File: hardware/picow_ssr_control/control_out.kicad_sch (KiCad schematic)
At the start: 12 parts

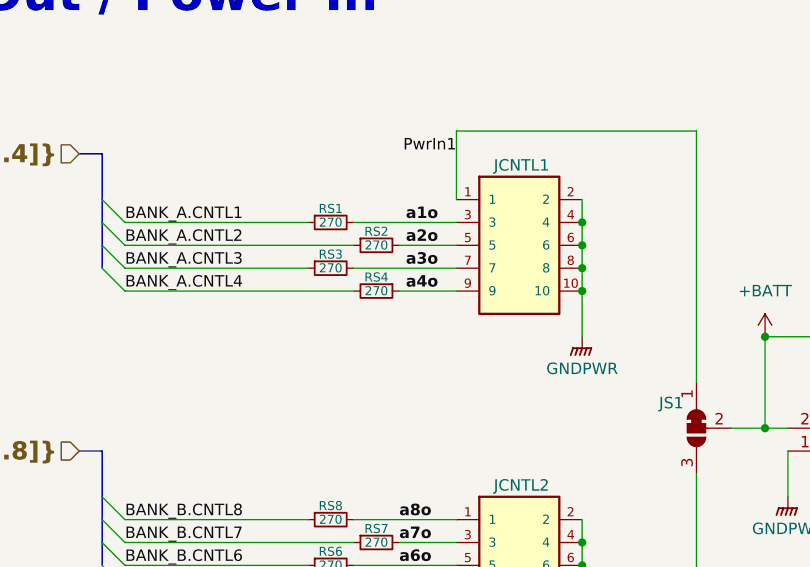
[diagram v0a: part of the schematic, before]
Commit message: Updated schemas
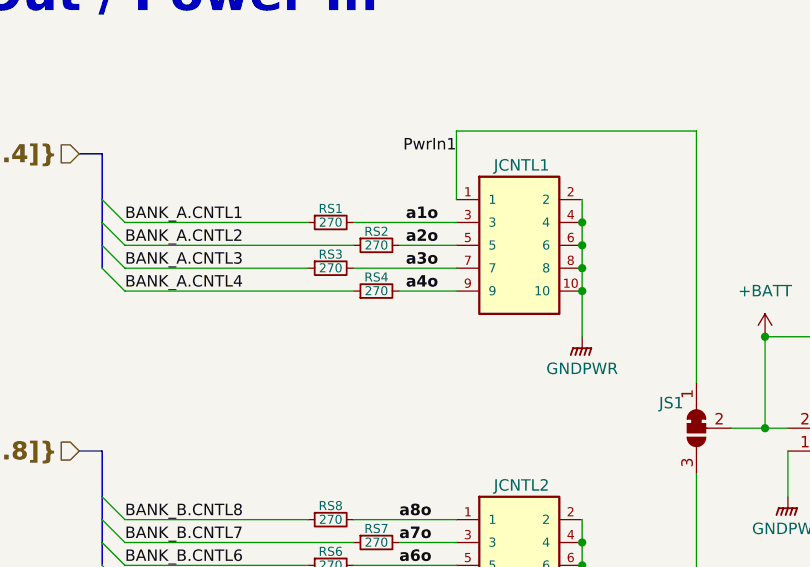
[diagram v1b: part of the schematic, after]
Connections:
- net BANK_A.CNTL4: now also RS4.1; no longer RS4.2
- net a4o: now also RS4.2; no longer RS4.1
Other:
- moved on the sheet: RS4
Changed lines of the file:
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@@
   (paper "USLetter")
   (title_block
-    (date "2023-01-27")
+    (date "2023-01-28")
     (rev "0.0.10")
     (comment 2 "http://creativecommons.org/licenses/by-sa/4.0/")
@@
   )
   (bus (pts (xy 53.34 68.58) (xy 53.34 73.66))
-    (stroke (width 0) (type default) (color 0 0 0 0))
+    (stroke (width 0) (type default) (color 255 255 0 1))
   )
   (wire (pts (xy 119.38 33.02) (xy 92.71 33.02))
@@
   )
   (bus (pts (xy 53.34 40.64) (xy 53.34 43.18))
-    (stroke (width 0) (type default) (color 0 0 0 0))
+    (stroke (width 0) (type default) (color 255 255 0 1))
   )
   (wire (pts (xy 92.71 33.02) (xy 92.71 40.64))
@@
   )
   (bus (pts (xy 53.34 43.18) (xy 53.34 45.72))
-    (stroke (width 0) (type default) (color 0 0 0 0))
+    (stroke (width 0) (type default) (color 255 255 0 1))
   )
   (wire (pts (xy 92.71 91.44) (xy 92.71 86.36))
@@
   )
   (bus (pts (xy 53.34 73.66) (xy 53.34 76.2))
+    (stroke (width 0) (type default) (color 255 255 0 1))
+  )
+  (wire (pts (xy 81.28 48.26) (xy 92.71 48.26))
     (stroke (width 0) (type default) (color 0 0 0 0))
   )
@@
   )
   (bus (pts (xy 50.8 35.56) (xy 53.34 35.56))
-    (stroke (width 0) (type default) (color 0 0 0 0))
+    (stroke (width 0) (type default) (color 255 255 0 1))
   )
   (bus (pts (xy 50.8 68.58) (xy 53.34 68.58))
-    (stroke (width 0) (type default) (color 0 0 0 0))
+    (stroke (width 0) (type default) (color 255 255 0 1))
   )
   (wire (pts (xy 55.88 48.26) (xy 76.2 48.26))
@@
   )
   (bus (pts (xy 53.34 45.72) (xy 53.34 48.26))
-    (stroke (width 0) (type default) (color 0 0 0 0))
+    (stroke (width 0) (type default) (color 255 255 0 1))
   )
   (wire (pts (xy 127 55.88) (xy 127 66.04))
@@
   )
   (bus (pts (xy 53.34 76.2) (xy 53.34 78.74))
-    (stroke (width 0) (type default) (color 0 0 0 0))
+    (stroke (width 0) (type default) (color 255 255 0 1))
   )
   (bus (pts (xy 53.34 35.56) (xy 53.34 40.64))
-    (stroke (width 0) (type default) (color 0 0 0 0))
+    (stroke (width 0) (type default) (color 255 255 0 1))
   )
   (wire (pts (xy 127 55.88) (xy 132.08 55.88))
@@
     (stroke (width 0) (type default) (color 0 0 0 0))
   )
-  (wire (pts (xy 92.71 48.26) (xy 81.28 48.26))
-    (stroke (width 0) (type default) (color 0 0 0 0))
-  )
   (wire (pts (xy 92.71 50.8) (xy 86.36 50.8))
     (stroke (width 0) (type default) (color 0 0 0 0))
@@
   )
   (bus (pts (xy 53.34 78.74) (xy 53.34 81.28))
-    (stroke (width 0) (type default) (color 0 0 0 0))
+    (stroke (width 0) (type default) (color 255 255 0 1))
   )
   (wire (pts (xy 106.68 50.8) (xy 106.68 55.88))
@@
     (pin "2")
   )
-  (symbol (lib_id "Device:R_Small") (at 83.82 50.8 270) (unit 1)
+  (symbol (lib_name "R_Small_1") (lib_id "Device:R_Small") (at 83.82 50.8 90) (unit 1)
     (in_bom yes) (on_board yes)
     (property "Reference" "RS4" (id 0) (at 83.82 49.276 90)
@@
     (pin "1")
   )
-  (symbol (lib_id "Device:R_Small") (at 83.82 83.82 90) (mirror x) (unit 1)
+  (symbol (lib_name "R_Small_2") (lib_id "Device:R_Small") (at 83.82 83.82 90) (mirror x) (unit 1)
     (in_bom yes) (on_board yes)
     (property "Reference" "RS5" (id 0) (at 83.82 82.296 90)
